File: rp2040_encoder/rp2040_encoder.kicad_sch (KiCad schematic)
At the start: 25 parts, among them J1 Conn_01x05, U1 SN74LVC1G07QDCKTQ1, U2 SN74LVC1G07QDCKTQ1, U3 SN74LVC1G79DBVR, U4 SN74LVC1G07QDCKTQ1, U5 MT6701

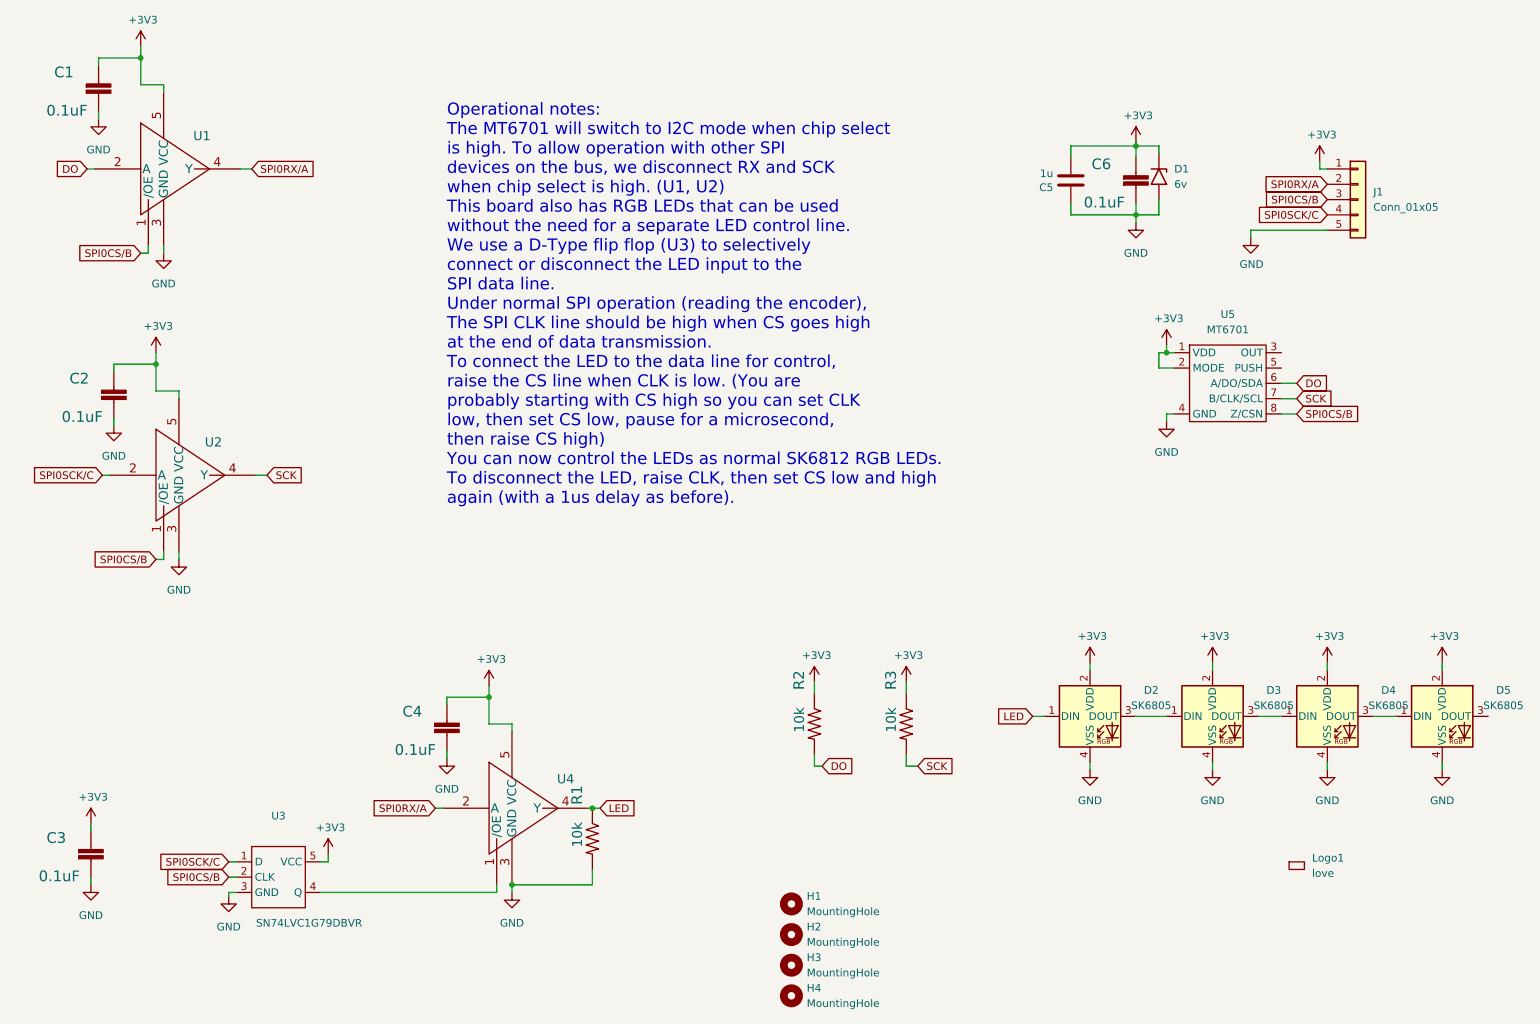
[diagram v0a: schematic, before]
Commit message: Update boards for latest build, pending design review.
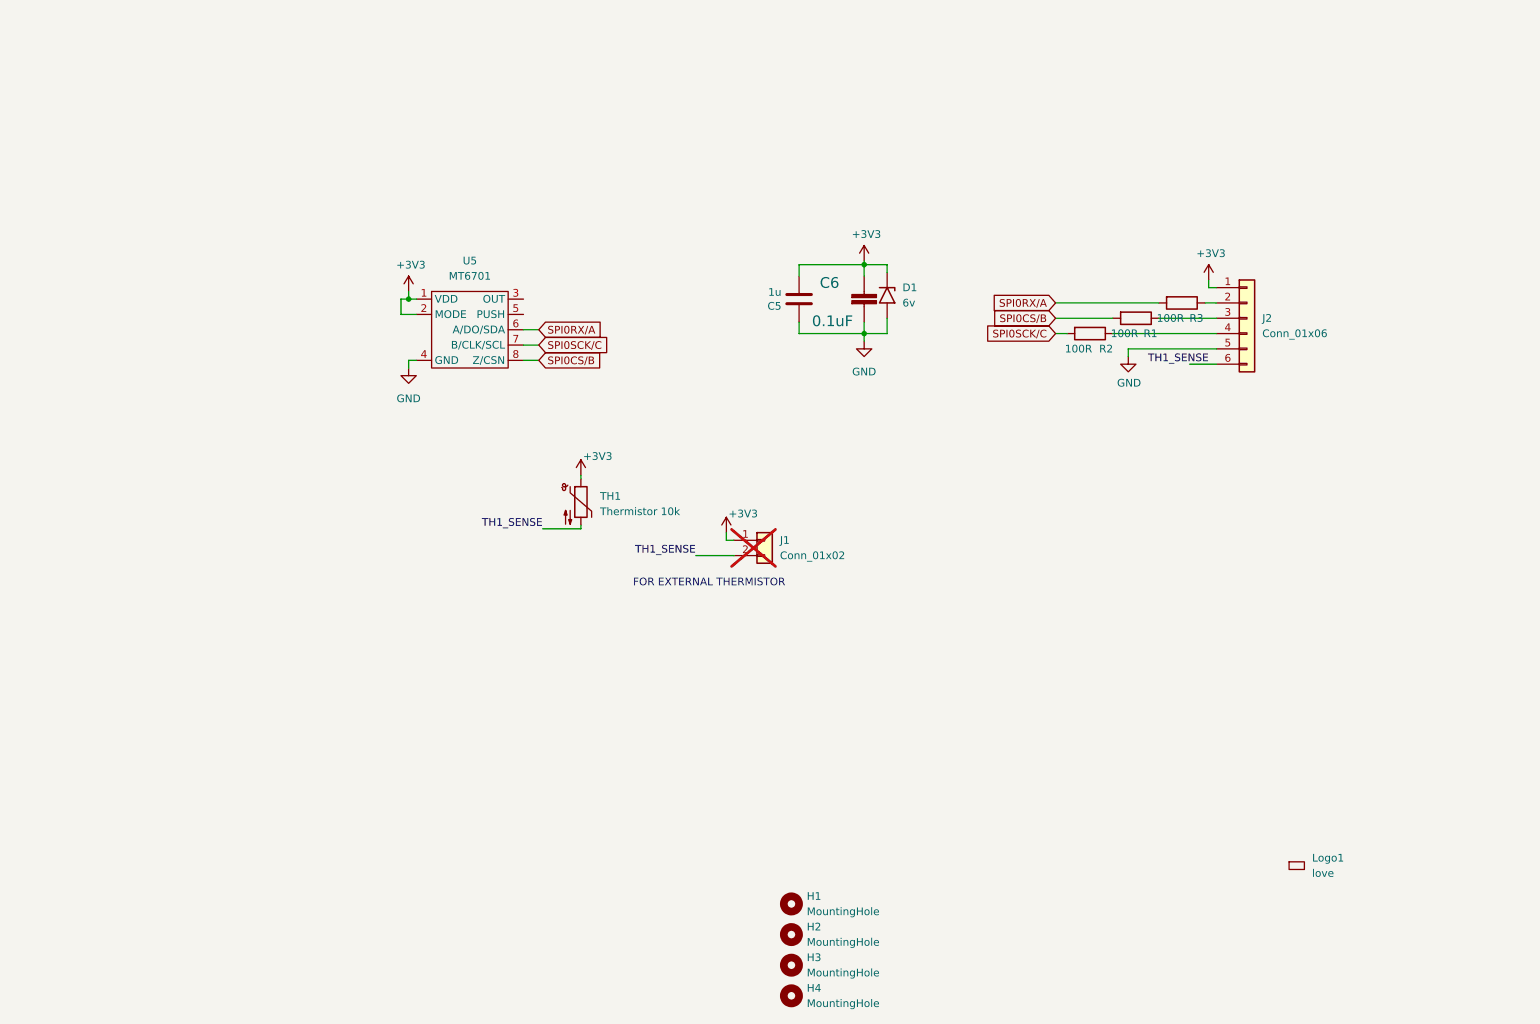
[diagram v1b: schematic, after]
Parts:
- removed C1, C2, C3, C4: 0.1uF, Capacitor_SMD:C_0603_1608Metric, symbol MotorController:SPARKFUN-CAPACITORS_CAP
- removed D2, D3, D4, D5: SK6805, LED_SMD:LED_SK6812_EC15_1.5x1.5mm, symbol encoder_parts:SK6805-EC15
- removed J1: Conn_01x05, parts:Molex_KK-254_1x05_P2.54mm_Horizontal, symbol Connector_Generic:Conn_01x05
- removed R1, R2, R3: 10k, Resistor_SMD:R_0603_1608Metric, symbol MotorController:TAYLOR_RESISTOR
- removed U1, U2, U4: SN74LVC1G07QDCKTQ1, Package_TO_SOT_SMD:SOT-353_SC-70-5, symbol acorn-motherboard:SN74LVC1G07QDCKTQ1
- removed U3: SN74LVC1G79DBVR, Package_TO_SOT_SMD:SOT-353_SC-70-5, symbol encoder_parts:SN74LVC1G80DCKR
- added J1: Conn_01x02, Connector_PinHeader_2.54mm:PinHeader_1x02_P2.54mm_Vertical, symbol Connector_Generic:Conn_01x02
- added J2: Conn_01x06, parts:Molex_KK-254_1x06_P2.54mm_Horizontal, symbol Connector_Generic:Conn_01x06
- added R1, R2, R3: 100R, Resistor_SMD:R_0603_1608Metric, symbol Device:R
- added TH1: Thermistor 10k, Resistor_SMD:R_0603_1608Metric, symbol Device:Thermistor_NTC
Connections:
- net DO is gone; now on net SPI0RX/A: U5.6 (A/DO/SDA)
- net SCK is gone; now on net SPI0SCK/C: U5.7 (B/CLK/SCL)
- net +3V3: now also J1.1 (Pin_1), J2.1 (Pin_1), TH1.1
- net GND: now also J2.5 (Pin_5)
- net SPI0CS/B: now also R1.2
- net SPI0RX/A: now also R3.2
- net SPI0SCK/C: now also R2.2
- new net: J2.4 (Pin_4), R2.1
- new net: J2.2 (Pin_2), R3.1
- new net: J2.3 (Pin_3), R1.1
- new net TH1_SENSE: J1.2 (Pin_2), J2.6 (Pin_6), TH1.2
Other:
- note added: "FOR EXTERNAL THERMISTOR"
- note removed: "Operational notes: The MT6701 will switch to I2C mode when chip select is high. To allow operation with other SPI devices on the bus, we disconnect RX and SCK when chip select is high. (U1, U2) This board also has RGB LEDs that can be used without the need for a separate LED control line. We use a D-Type flip flop (U3) to selectively connect or disconnect the LED input to the SPI data line. Under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"
- moved on the sheet: C5, C6, D1, U5
